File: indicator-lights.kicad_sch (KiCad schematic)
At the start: 17 parts, among them IC7 LP55231SQX_NOPB

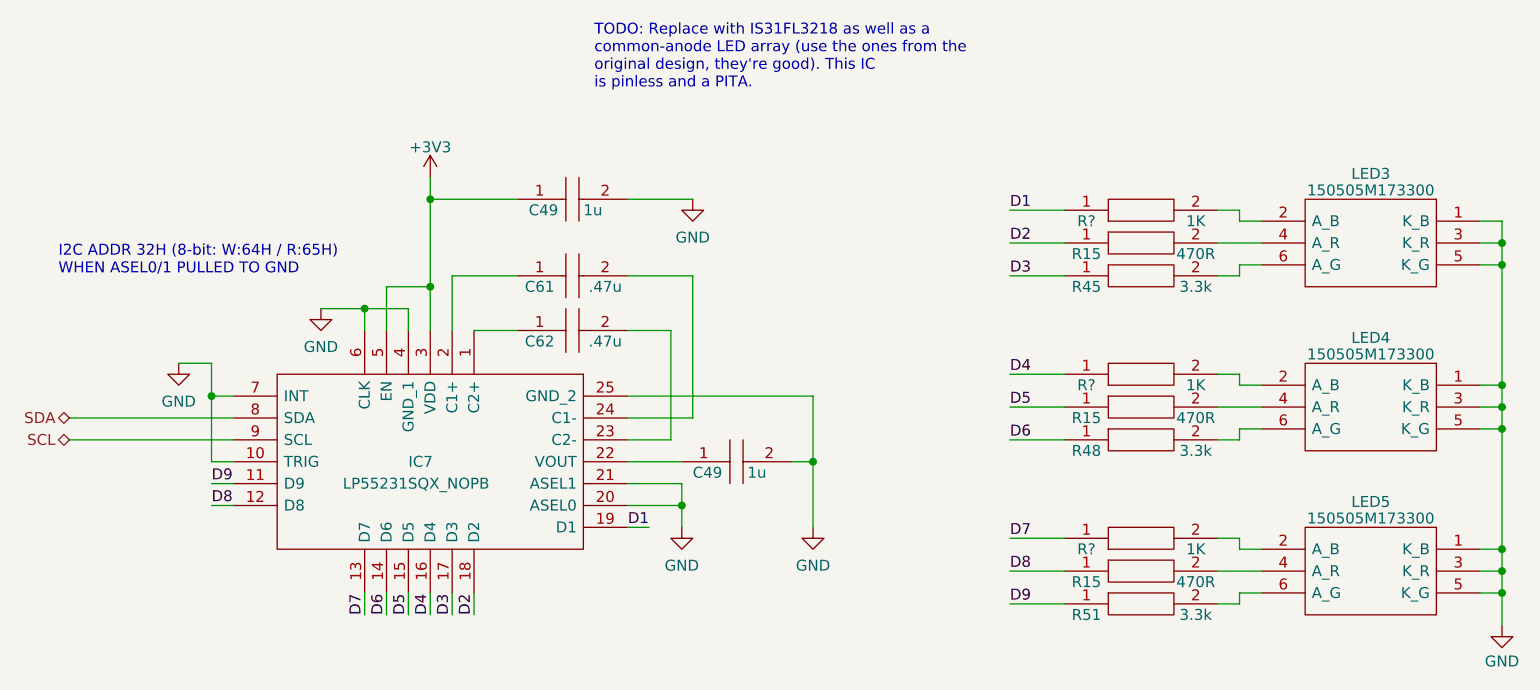
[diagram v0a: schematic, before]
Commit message: first round of revisions
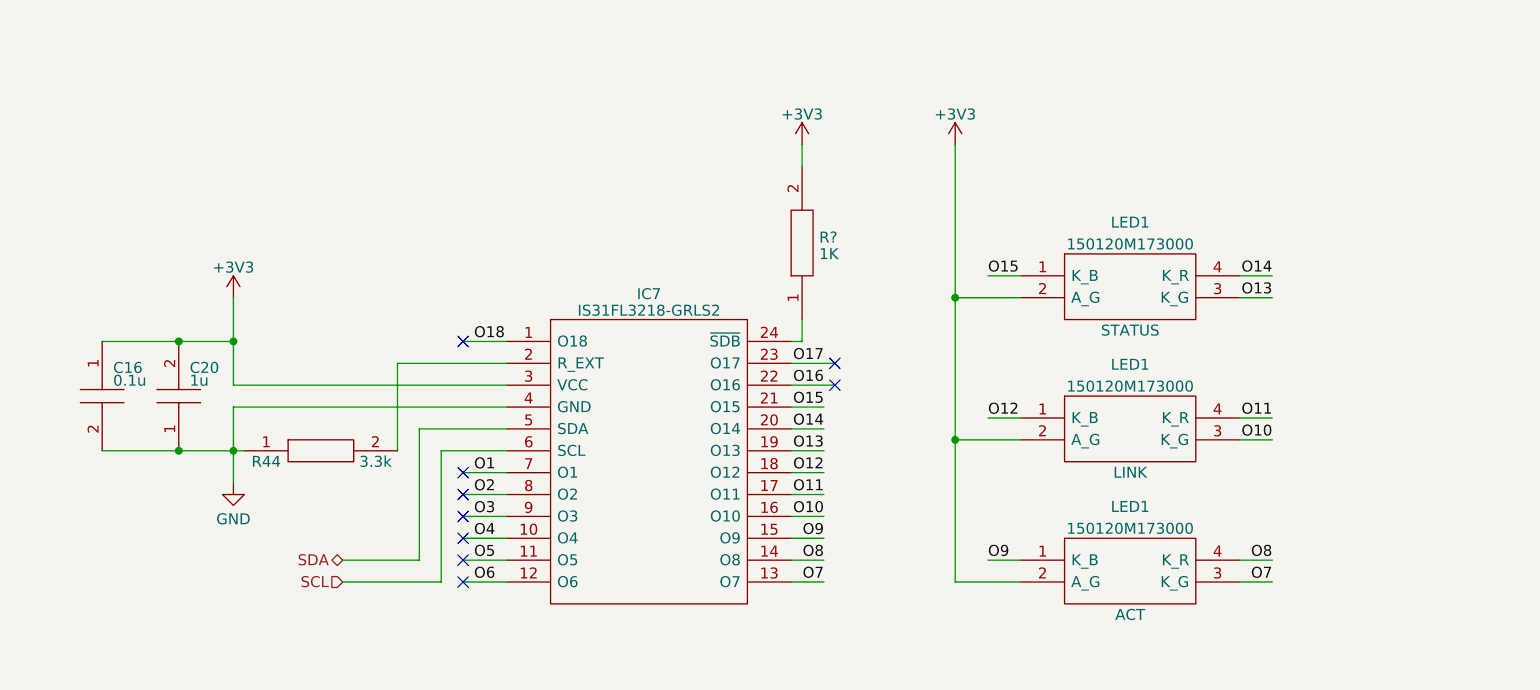
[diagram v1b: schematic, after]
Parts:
- removed C49 (x2): 1u, CAPC1608X90N, symbol SamacSys_Parts:0603YD105KAT2A
- removed C61, C62: .47u, CAPC0603X33N, symbol SamacSys_Parts:LMK063BC6474KPLF
- removed IC7: LP55231SQX_NOPB, SamacSys_Parts:QFN50P400X400X80-25N, symbol SamacSys_Parts:LP55231SQX_NOPB
- removed LED3, LED4, LED5: 150505M173300, 150505M173300, symbol SamacSys_Parts:150505M173300
- removed R15 (x3): 470R, RESC2012X60N, symbol SamacSys_Parts:AC0805FR-07470RL
- removed R45, R48, R51: 3.3k, RESC1608X55N, symbol SamacSys_Parts:RC0603JR-133K3L
- removed R? (x3): 1K, SamacSys_Parts:RESC2012X60N, symbol SamacSys_Parts:SG73P2ATTD102J
- added C16: 0.1u, SamacSys_Parts:CAPC0402X22N, symbol SamacSys_Parts:01016D104KAT2A
- added C20: 1u, SamacSys_Parts:CAPC1608X90N, symbol SamacSys_Parts:0603YD105KAT2A
- added IC7: IS31FL3218-GRLS2, SOIC127P1036X265-24N, symbol SamacSys_Parts:IS31FL3218-GRLS2
- added LED1 (x3): 150120M173000, 150120M173000, symbol SamacSys_Parts:150120M173000
- added R44: 3.3k, RESC1608X55N, symbol SamacSys_Parts:RC0603JR-133K3L
- added R?: 1K, SamacSys_Parts:RESC2012X60N, symbol SamacSys_Parts:SG73P2ATTD102J
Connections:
- net +3V3: now also C16.1, C20.2, IC7.3 (VCC), LED1.2 (A_G), LED1.2 (A_G), LED1.2 (A_G), R?.2
- net GND: now also C16.2, C20.1, IC7.4 (GND), R44.1
- net SCL: now also IC7.6 (SCL)
- net SDA: now also IC7.5 (SDA)
- new net: IC7.2 (R_EXT), R44.2
- new net: IC7.24 (~{SDB}), R?.1
- new net O1: IC7.7 (O1)
- new net O10: IC7.16 (O10), LED1.3 (K_G)
- new net O11: IC7.17 (O11), LED1.4 (K_R)
- new net O12: IC7.18 (O12), LED1.1 (K_B)
- new net O13: IC7.19 (O13), LED1.3 (K_G)
- new net O14: IC7.20 (O14), LED1.4 (K_R)
- new net O15: IC7.21 (O15), LED1.1 (K_B)
- new net O16: IC7.22 (O16)
- new net O17: IC7.23 (O17)
- new net O18: IC7.1 (O18)
- new net O2: IC7.8 (O2)
- new net O3: IC7.9 (O3)
- new net O4: IC7.10 (O4)
- new net O5: IC7.11 (O5)
- new net O6: IC7.12 (O6)
- new net O7: IC7.13 (O7), LED1.3 (K_G)
- new net O8: IC7.14 (O8), LED1.4 (K_R)
- new net O9: IC7.15 (O9), LED1.1 (K_B)
- no-connect marks 0 -> 9
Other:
- note removed: "I2C ADDR 32H (8-bit: W:64H / R:65H) WHEN ASEL0/1 PULLED TO GND"
- note removed: "TODO: Replace with IS31FL3218 as well as a common-anode LED array (use the ones from the original design, they're good). This IC is pinless and a PITA."
